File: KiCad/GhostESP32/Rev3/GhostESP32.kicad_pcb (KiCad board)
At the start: 2 copper layers, 60 x 37 mm, 44 parts, among them J1 CONN_02X20, P1 USB_OTG, Q1 Q_NPN_BEC, Q2 Q_NPN_BEC, Q3 Q_NPN_BEC, SW1 SW_SPDT, U1 LM358, U2 NCP1117ST33T3G, U3 CP2102, U4 ESP-WROOM-32, U5 MPU-6050, U6 HMC5883

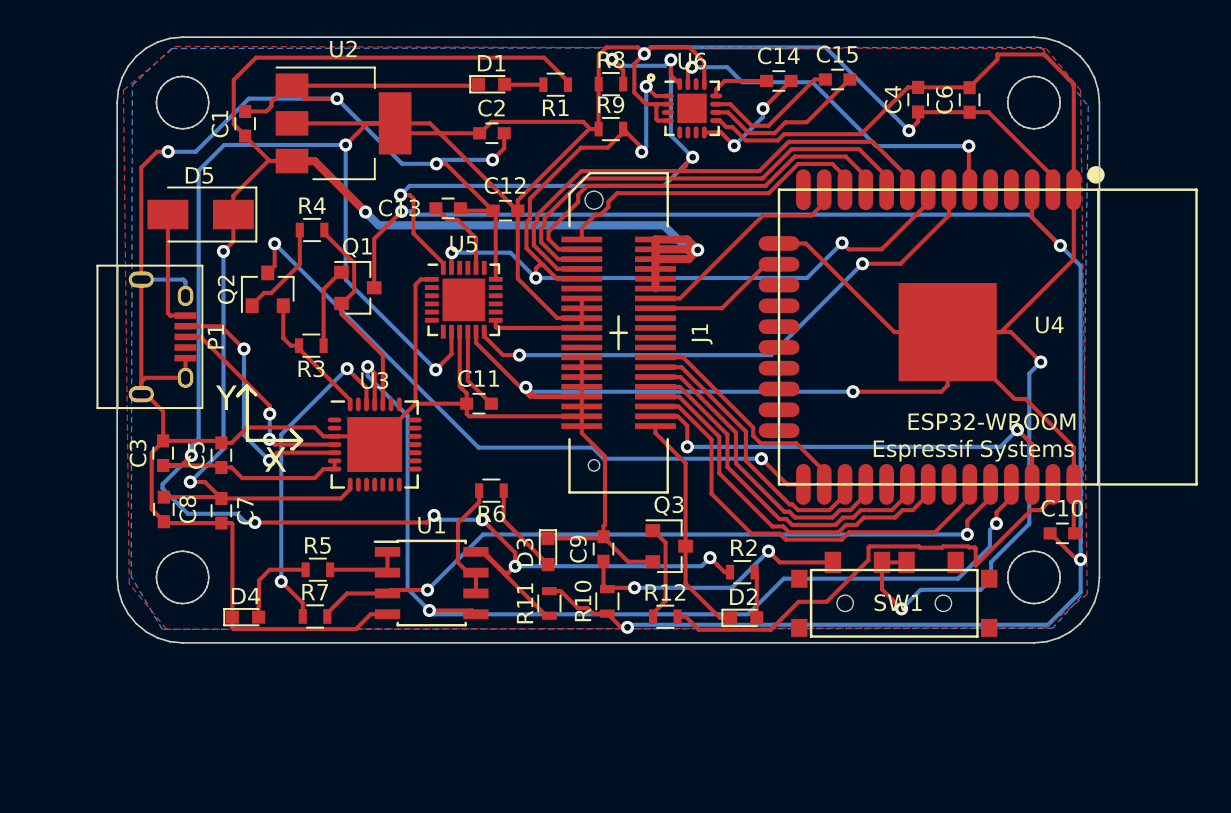
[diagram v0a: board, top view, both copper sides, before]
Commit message: Working on Rev3 of GhostESP32
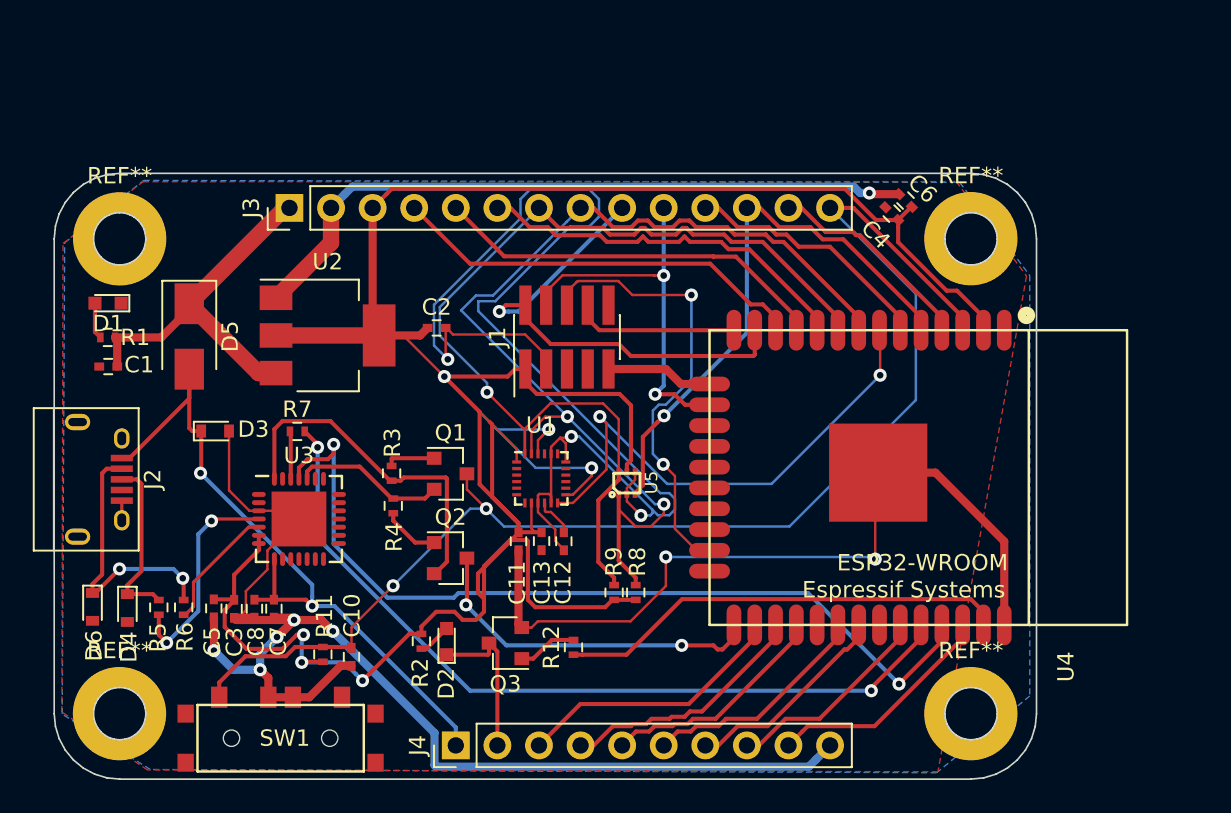
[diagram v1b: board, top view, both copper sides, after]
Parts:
- removed C14: 0.22uF, Capacitors_SMD:C_0603
- removed C15: 4.7uF, Capacitors_SMD:C_0603
- removed C9: 1nF, Capacitors_SMD:C_0603
- removed P1: USB_OTG, Connectors:USB_Micro-B
- removed R10: 470, Resistors_SMD:R_0603
- removed U6: HMC5883, Housings_DFN_QFN:QFN-16-1EP_3x3mm_Pitch0.5mm
- added D6: ESD, Diodes_SMD:D_0603, F.Cu at (115.5, 105.5)
- added J2: USB_OTG, Connectors:USB_Micro-B, F.Cu at (115.9, 97.7)
- added J3: CONN_01X14, Pin_Headers:Pin_Header_Straight_1x14_Pitch2.54mm, F.Cu at (127.5, 81.2)
- added J4: CONN_01X10, Pin_Headers:Pin_Header_Straight_1x10_Pitch2.54mm, F.Cu at (137.7, 114.0)
- added REF**: MountingHole_3.2mm_M3_ISO7380_Pad, Mounting_Holes:MountingHole_3.2mm_M3_ISO7380_Pad, F.Cu at (117.1, 112.0)
- added REF**: MountingHole_3.2mm_M3_ISO7380_Pad, Mounting_Holes:MountingHole_3.2mm_M3_ISO7380_Pad, F.Cu at (117.1, 83.0)
- added REF**: MountingHole_3.2mm_M3_ISO7380_Pad, Mounting_Holes:MountingHole_3.2mm_M3_ISO7380_Pad, F.Cu at (169.1, 112.0)
- added REF**: MountingHole_3.2mm_M3_ISO7380_Pad, Mounting_Holes:MountingHole_3.2mm_M3_ISO7380_Pad, F.Cu at (169.1, 83.0)
- C1, C11, C2, C3, C4, C5, C6, C7, C8: footprint Capacitors_SMD:C_0603 -> Capacitors_SMD:C_0402
- C10: value 1nF -> 1uF; footprint Capacitors_SMD:C_0603 -> Capacitors_SMD:C_0402
- C12: value 10nF -> 0.1uF; footprint Capacitors_SMD:C_0603 -> Capacitors_SMD:C_0402
- C13: value 2.2nF -> 10nF; footprint Capacitors_SMD:C_0603 -> Capacitors_SMD:C_0402
- D1: value RED LED -> GREEN LED
- D3: value RXLED -> ESD; footprint LEDs:LED_0603 -> Diodes_SMD:D_0603
- D4: value TXLED -> ESD; footprint LEDs:LED_0603 -> Diodes_SMD:D_0603
- D5: footprint Diodes_SMD:D_SMA_Standard -> Diodes_SMD:D_SMA
- J1: value CONN_02X20 -> CONN_02X05; footprint hrs-fx8c:hrs-fx8c-40p-sv -> Pin_Headers:Pin_Header_Straight_2x05_Pitch1.27mm_SMD
- R1, R11, R12, R2, R3, R4, R7, R8, R9: footprint Resistors_SMD:R_0603 -> Resistors_SMD:R_0402
- R5, R6: value 1k -> 68; footprint Resistors_SMD:R_0603 -> Resistors_SMD:R_0402
- U1: value LM358 -> MPU-9250; footprint Housings_SOIC:SOIC-8_3.9x4.9mm_Pitch1.27mm -> Housings_DFN_QFN:QFN-24_3x3mm_Pitch0.4mm
- U5: value MPU-6050 -> TMP102; footprint Housings_DFN_QFN:QFN-24-1EP_4x4mm_Pitch0.5mm -> NorBotKiCadFootprints:SOT563
- moved C10 44.1 mm to (131.3, 108.6), turned to 270 degrees
- moved SW1 38.4 mm to (127.0, 113.5)
- moved R1 31.4 mm to (116.4, 89.1)
- moved R8 31.1 mm to (148.6, 104.6), turned to 90 degrees
- moved R9 28.3 mm to (147.3, 104.6), turned to 90 degrees
- moved D1 27.0 mm to (116.4, 87.0), turned to 180 degrees
- moved D3 21.6 mm to (123.0, 94.8), turned to 0 degrees
- moved C13 21.1 mm to (142.9, 101.5), turned to 270 degrees
- moved C12 20.5 mm to (144.2, 101.5), turned to 270 degrees
- moved R6 20.1 mm to (121.0, 105.5), turned to 90 degrees
- moved R2 20.1 mm to (135.6, 107.6), turned to 90 degrees
- moved Q2 19.9 mm to (137.3, 102.5), turned to 0 degrees
- moved D2 18.2 mm to (137.1, 107.6), turned to 90 degrees
- moved R4 17.6 mm to (133.8, 99.3), turned to 90 degrees
- moved C1 17.0 mm to (116.4, 90.8), turned to 180 degrees
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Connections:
- C1 pad 1: +5V -> +BATT
- C11 pad 1: GND -> +3V3
- C11 pad 2: Net-(C11-Pad2) -> GND
- C12 pad 1: GND -> Net-(C12-Pad1)
- C12 pad 2: +3V3 -> GND
- C13 pad 1: GND -> +3V3
- C13 pad 2: Net-(C13-Pad2) -> GND
- C7 pad 1: +5V -> VBUS
- C8 pad 1: +5V -> VBUS
- D3 pad 1: GND -> VBUS
- D3 pad 2: Net-(D3-Pad2) -> GND
- D4 pad 1: GND -> Net-(D4-Pad1)
- D4 pad 2: Net-(D4-Pad2) -> GND
- D5 pad 1: +5V -> +BATT
- D5 pad 2: Net-(D5-Pad2) -> VBUS
- J1 pad 1: IO27 -> +3V3
- J1 pad 10: +3V3 -> (no net)
- J1 pad 2: IO26 -> IO14
- J1 pad 3: IO25 -> GND
- J1 pad 4: IO33 -> IO13
- J1 pad 5: IO32 -> GND
- J1 pad 6: (no net) -> IO15
- J1 pad 7: +3V3 -> GND
- J1 pad 8: +3V3 -> IO12
- J1 pad 9: +3V3 -> GND
- R1 pad 1: +5V -> +BATT
- R12 pad 1: Net-(Q3-Pad1) -> IO23
- R12 pad 2: IO23 -> Net-(Q3-Pad1)
- R5 pad 1: Net-(D4-Pad2) -> USB_DP
- R5 pad 2: Net-(R5-Pad2) -> Net-(D4-Pad1)
- R6 pad 1: Net-(D3-Pad2) -> USB_DN
- R6 pad 2: Net-(R6-Pad2) -> Net-(D6-Pad1)
- R8 pad 2: IO33 -> IO32/SCL
- R9 pad 2: IO32 -> IO33/SDA
- SW1 pad 3: Net-(C9-Pad1) -> EN
- U1 pad 1: Net-(R5-Pad2) -> +3V3
- U1 pad 2: Net-(R5-Pad2) -> (no net)
- U1 pad 3: TXD -> (no net)
- U1 pad 4: GND -> (no net)
- U1 pad 5: RXD -> (no net)
- U1 pad 6: Net-(R6-Pad2) -> (no net)
- U1 pad 7: Net-(R6-Pad2) -> (no net)
- U2 pad 3: +5V -> +BATT
- U3 pad 8: +5V -> VBUS
- U4 pad 14: (no net) -> IO12
- U4 pad 23: (no net) -> IO15
- U4 pad 4: (no net) -> I36
- U4 pad 5: (no net) -> I39
- U4 pad 6: IO34 -> I34
- U4 pad 7: IO35 -> I35
- U4 pad 8: IO32 -> IO32/SCL
- U4 pad 9: IO33 -> IO33/SDA
- U5 pad 1: GND -> IO32/SCL
- U5 pad 2: (no net) -> GND
- U5 pad 3: (no net) -> I39
- U5 pad 4: (no net) -> GND
- U5 pad 5: (no net) -> +3V3
- U5 pad 6: (no net) -> IO33/SDA
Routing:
- net +5V: track 105.1 -> 0.00 mm, vias 4 -> 0
- net IO33: track 71.3 -> 0.00 mm, vias 4 -> 0
- net GND: track 321.5 -> 256.7 mm, vias 8 -> 11
- net IO32/SCL: track 0.00 -> 63.4 mm, vias 0 -> 2
- net IO33/SDA: track 0.00 -> 61.5 mm, vias 0 -> 1
- net IO32: track 57.2 -> 0.00 mm, vias 5 -> 0
- net VBUS: track 0.00 -> 44.5 mm, vias 0 -> 2
- net I39: track 0.00 -> 34.5 mm, vias 0 -> 1
- net IO35: track 34.2 -> 0.00 mm, vias 2 -> 0
- net +3V3: track 215.9 -> 184.1 mm, vias 10 -> 6
- net I35: track 0.00 -> 31.6 mm, vias 0 -> 2
- net EN: track 109.0 -> 80.5 mm, vias 4 -> 2
- net IO15: track 0.00 -> 27.8 mm, vias 0 -> 2
- net +BATT: track 0.00 -> 23.0 mm
- net IO34: track 22.7 -> 0.00 mm, vias 2 -> 0
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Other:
- net class POWER added: clearance 0.2, trace_width 0.5, via_dia 0.8, via_drill 0.4
- net class THIN added: clearance 0.2, trace_width 0.2, via_dia 0.8, via_drill 0.4
- rule trace_min: 0.2 -> 0.15
- board text removed: "Ghost ESP32, rev 2 Frode Lillerud 19.mar 2017"
- board text removed: "X"
- board text removed: "Y"
